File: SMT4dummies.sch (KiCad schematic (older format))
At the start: 0 parts

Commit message: Merged both sides
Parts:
- added C1: CP1, symbol CP1
- added C2: 0.1uF, symbol C
- added D1, D10, D11, D12, D2, D3, D4, D5, D6, D7, D8, D9: LED, symbol LED
- added D13, D14: 1N4148, symbol DIODE
- added IC1: 4520, symbol 4520
- added IC2: LM2902N, symbol LM2902N
- added IC3: LM555N, symbol LM555N
- added J1: USB_2, symbol USB_2
- added P1: CONN_2, symbol CONN_2
- added Q1, Q2, Q3, Q4: NPN, symbol NPN
- added R1, R10, R11, R12, R13, R14, R15, R16, R17, R18, R19, R2, R20, R21, R22, R23, R3, R4, R5, R6: R, symbol R
- added R24, R25: 1K, symbol R
- added R8, R9: 4.7K, symbol R
- added RV1: POT, symbol POT
- added RV2: 100K, symbol POT
- added SW1, SW2, SW3, SW4: SW_PUSH, symbol SW_PUSH
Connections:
- new net: D7.1 (A), IC1.3 (Q1)
- new net: D6.1 (A), IC1.4 (Q2)
- new net: D5.1 (A), IC1.5 (Q3)
- new net: D4.1 (A), IC1.6 (Q4)
- new net: D4.2 (K), R10.1
- new net: D5.2 (K), R11.1
- new net: D7.2 (K), R13.1
- new net: D6.2 (K), R12.1
- new net: D8.1 (A), IC2.1
- new net: IC2.2 (-), R14.2, R15.1
- new net: IC2.6 (-), R15.2, R16.1
- new net: D9.1 (A), IC2.7
- new net: D10.1 (A), IC2.8
- new net: IC2.9 (-), R16.2, R17.1
- new net: IC2.13 (-), R17.2, R18.1
- new net: D11.1 (A), IC2.14
- new net: D8.2 (K), R19.2
- new net: D9.2 (K), R20.2
- new net: D11.2 (K), R22.2
- new net: D10.2 (K), R21.2
- new net: IC3.3 (Q), R25.2
- new net: D13.2 (K), RV2.1
- new net: D14.1 (A), RV2.3
- new net: Q4.2 (B), R25.1
- new net: Q4.3 (C), R23.2
- new net: D12.2 (K), R23.1
- new net: Q3.2 (B), R5.1, SW3.2
- new net: Q3.3 (C), R4.1, R6.2
- new net: Q2.2 (B), R4.2, SW2.2
- new net: Q2.3 (C), R3.2, R5.2
- new net: Q1.2 (B), R1.1
- new net: Q1.3 (C), R2.2
- new net: D3.2 (K), R6.1
- new net: D2.2 (K), R3.1
- new net: C1.1, R1.2, SW1.1
- new net: D1.2 (K), R2.1
- new net +5V: D1.1 (A), D12.1 (A), D2.1 (A), D3.1 (A), IC1.16 (VDD), IC1.2 (Enable), IC2.4 (V+), IC3.4 (R), IC3.8 (VCC), J1.1, P1.1 (P1), R14.1, R24.2, R8.2, RV1.1, SW1.2, SW4.1
- new net ANLG_INPUT: IC2.10 (+), IC2.12 (+), IC2.3 (+), IC2.5 (+), RV1.2
- new net CLK: IC1.1 (CK), R9.1, SW4.2
- new net DIS: IC3.7 (DIS), R24.1, RV2.2
- new net GND: C1.2, C2.2, IC1.7 (Reset), IC1.8 (VSS), IC2.11 (V-), IC3.1 (GND), IC3.5 (CV), J1.4, P1.2 (PM), Q1.1 (E), Q2.1 (E), Q3.1 (E), Q4.1 (E), R10.2, R11.2, R12.2, R13.2, R18.2, R19.1, R20.1, R21.1, R22.1, R8.1, R9.2, RV1.3, SW2.1, SW3.1
- new net THR: C2.1, D13.1 (A), D14.2 (K), IC3.2 (TR), IC3.6 (THR)
- no-connect marks 0 -> 2
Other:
- note added: "4 bits ADC"
- note added: "555-based PWM dimmer"
- note added: "KiCad needs this"
- note added: "Memory\n"
- note added: "Power supply"
- note added: "Push-switch operated 4-bit up binary counter"
- note added: "Time delay switch"

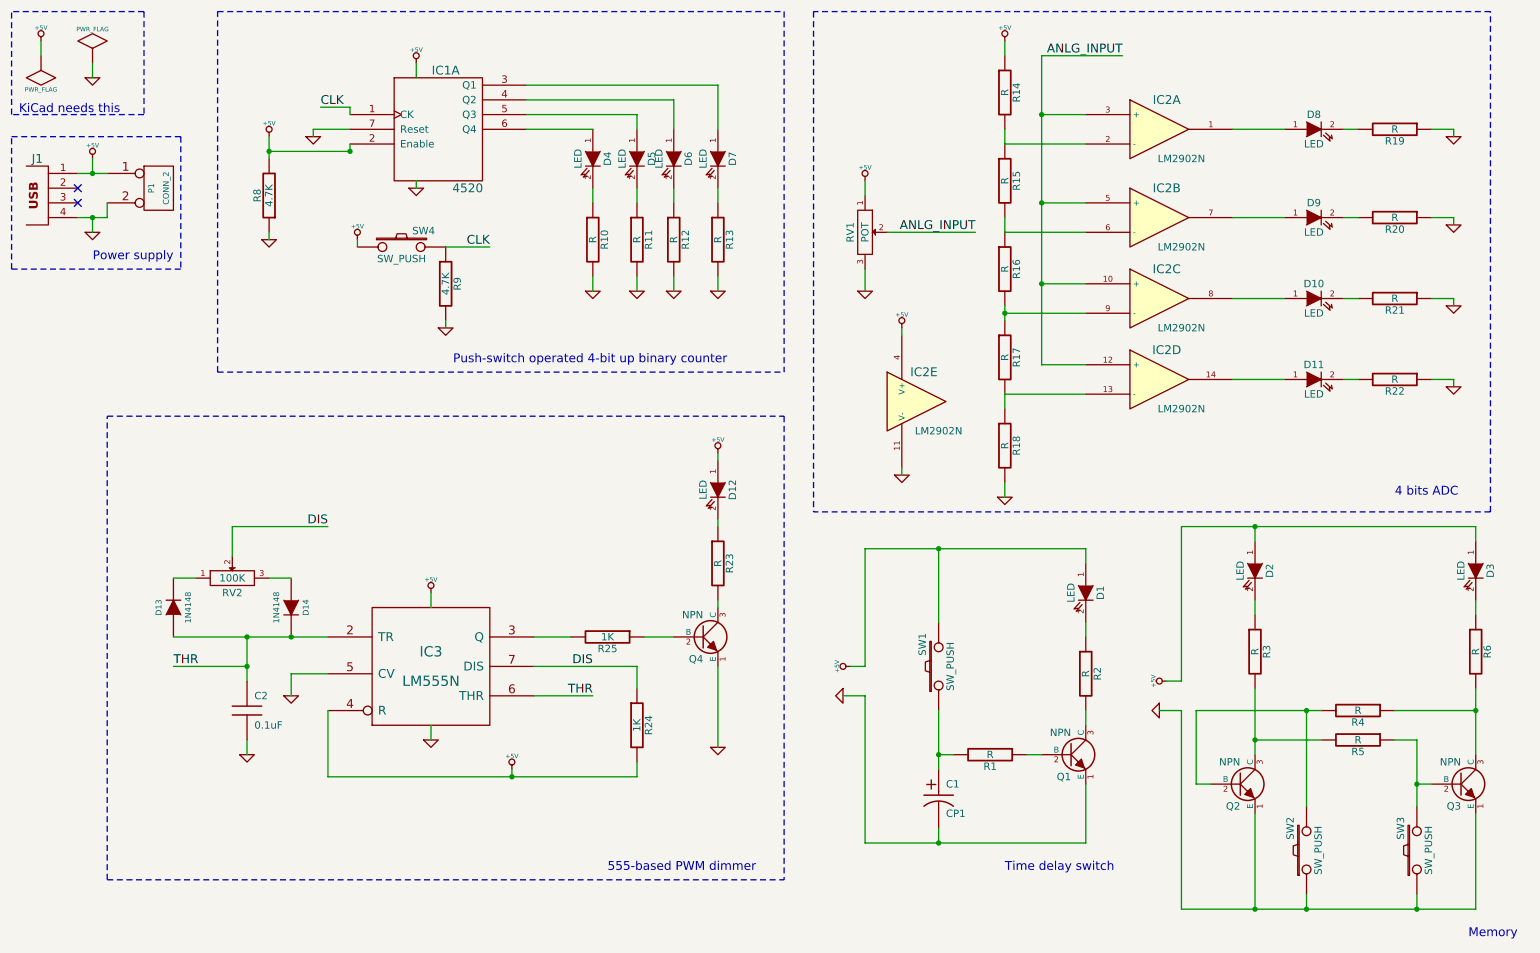
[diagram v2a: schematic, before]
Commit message: Modified counter.
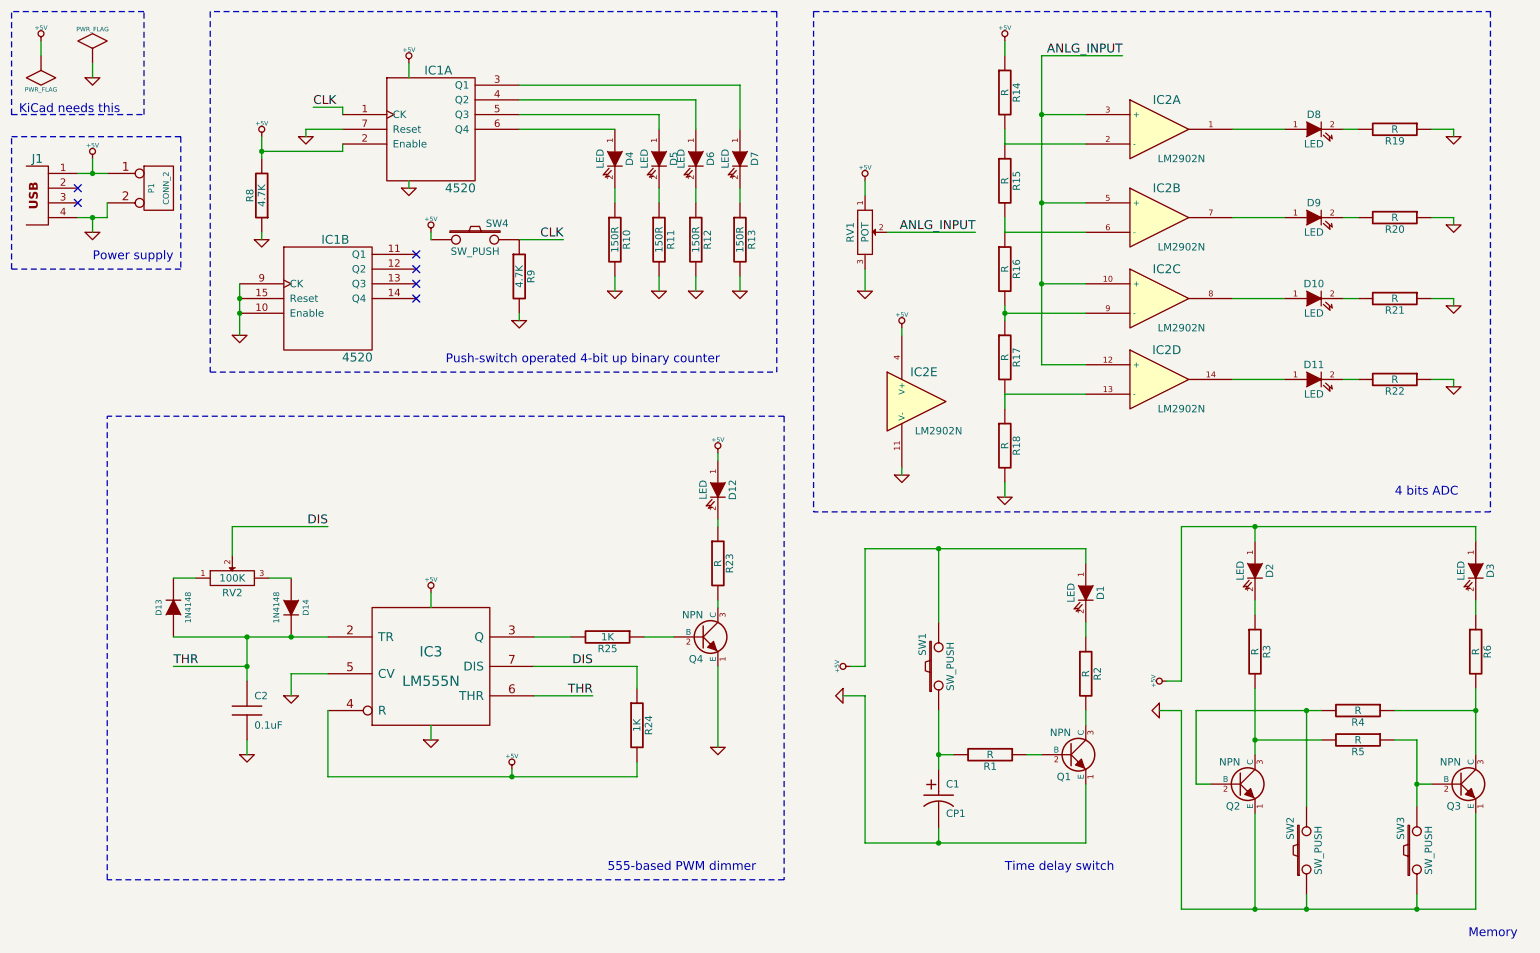
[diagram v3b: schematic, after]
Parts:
- added unit 2 of IC1
- R10, R11, R12, R13: value R -> 150R
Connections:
- net +5V: now also IC1.16 (VDD)
- net GND: now also IC1.10 (Enable), IC1.15 (Reset), IC1.8 (VSS), IC1.9 (CK)
- no-connect marks 2 -> 6
